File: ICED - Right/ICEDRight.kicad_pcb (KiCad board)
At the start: 2 copper layers, 175.4 x 145.5 mm, 162 parts, among them P1 FLASH_HDR, P2 USB3_MICRO, P3 CONN_17, P4 USB3_AFEMALE, Q1 TC1264, U1 MK20DX256VLH7, U2 IS31FL3731C, X1 CRYSTAL

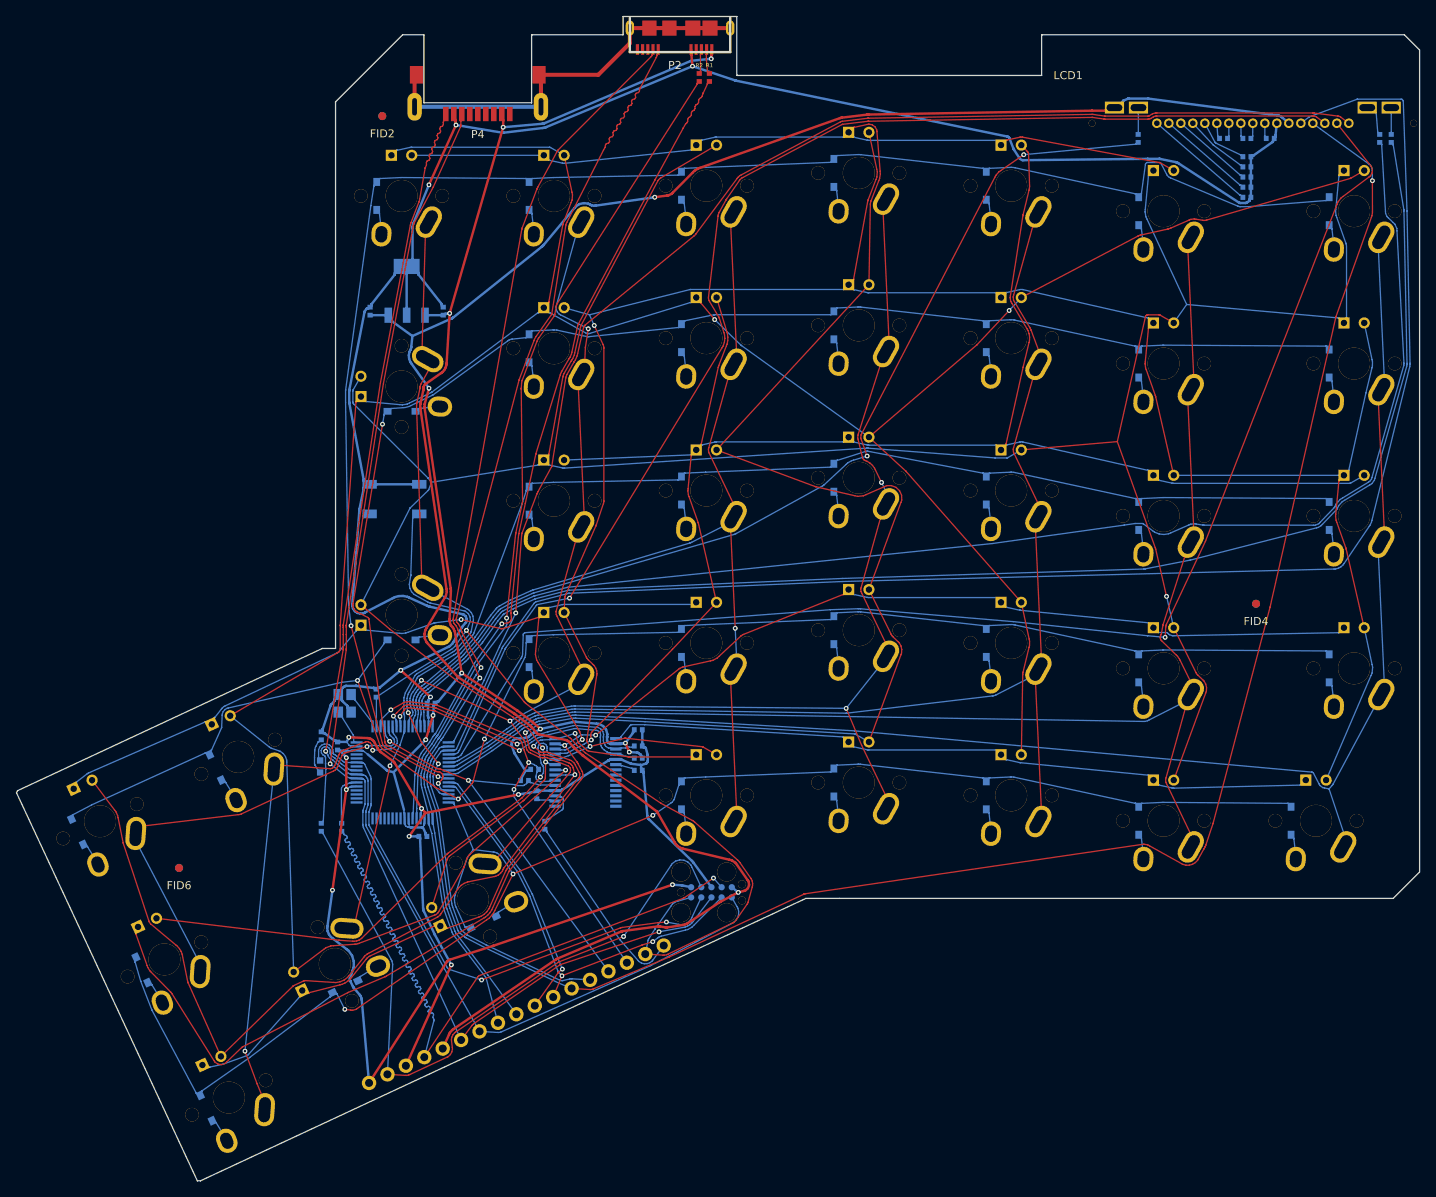
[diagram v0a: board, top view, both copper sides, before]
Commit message: ICED 1.2b, now with 100% more Type C
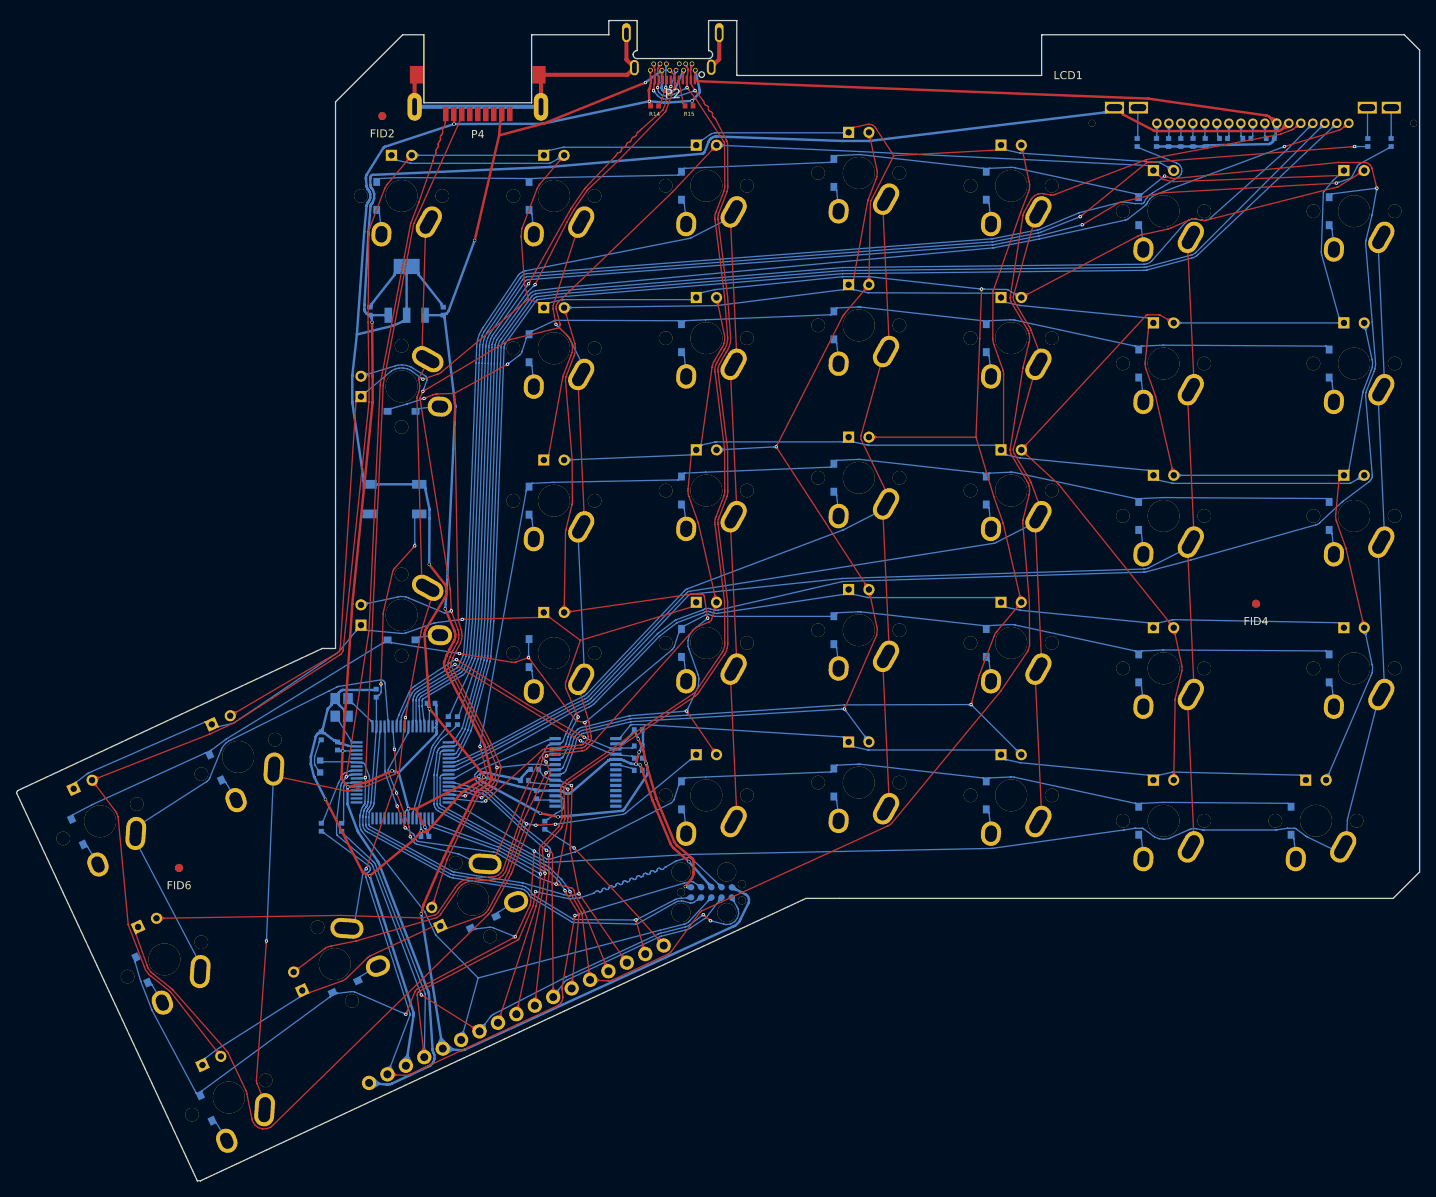
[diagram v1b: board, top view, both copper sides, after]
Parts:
- added R14: 5.1k, prettylib:SMD-1005, F.Cu at (104.0, 53.8)
- added R15: 5.1k, prettylib:SMD-1005, F.Cu at (108.3, 53.8)
- P2: value USB3_MICRO -> USBC; footprint prettylib:USB3_MICROB_STAKES -> prettylib:USB_C_MIDMOUNT_TH_IMPCUT
- R1, R2: moved to B.Cu
- moved R1 86.3 mm to (79.4, 130.7), turned to 180 degrees
- moved R2 86.3 mm to (78.2, 130.7), turned to 180 degrees
- moved C17 13.2 mm to (166.8, 58.4), turned to 0 degrees
- moved C16 11.3 mm to (168.3, 58.4), turned to 0 degrees
- moved C15 9.32 mm to (169.8, 58.4), turned to 0 degrees
- moved C14 7.39 mm to (171.3, 58.4), turned to 0 degrees
- moved P2 7.27 mm to (106.3, 49.9)
- moved C13 5.50 mm to (172.8, 58.4), turned to 0 degrees
- moved R10 1.57 mm to (193.2, 58.4)
- moved X1 0.64 mm to (64.9, 129.0)
- moved R13 0.52 mm to (164.3, 58.4)
- moved R9 0.51 mm to (196.1, 58.4)
- moved C4 0.25 mm to (75.3, 145.2)
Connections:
- net /mcu/PTB18 renamed /Col3
- net /mcu/PTB19 renamed /Col4
- net /mcu/PTB2 renamed /Col1
- net /mcu/PTB3 renamed /Col2
- net /mcu/PTC0 renamed /Col5
- net /mcu/PTC10 renamed /Col7
- net /mcu/PTC11 renamed /Col8
- net /mcu/PTC9 renamed /Col6
- net /mcu/PTD0 renamed /Col9
- net /mcu/PTD1 renamed /Row1
- net /mcu/PTD4 renamed /Row2
- net /mcu/PTD5 renamed /Row3
- net /mcu/PTD6 renamed /Row4
- net /mcu/PTD7 renamed /Row5
- P2 pad 1: +5V -> VSS
- P2 pad 10: (no net) -> /mcu/RX1
- P2 pad 11: /mcu/GND -> /mcu/TX1
- P2 pad 2: Net-(P2-Pad2) -> /mcu/TX1
- P2 pad 3: Net-(P2-Pad3) -> /mcu/RX1
- P2 pad 4: (no net) -> +5V
- P2 pad 5: VSS -> Net-(P2-Pad5)
- P2 pad 6: /mcu/RX1 -> /mcu/USB_DP
- P2 pad 7: /mcu/TX1 -> /mcu/USB_DM
- P2 pad 8: (no net) -> Net-(P2-Pad8)
- P2 pad 9: (no net) -> +5V
- P4 pad 10: /mcu/GND -> /GND
- P4 pad 2: (no net) -> Net-(P4-Pad2)
- P4 pad 3: (no net) -> Net-(P4-Pad3)
- P4 pad 7: (no net) -> Net-(P4-Pad7)
- P4 pad 8: (no net) -> Net-(P4-Pad8)
- P4 pad 9: (no net) -> Net-(P4-Pad9)
- R1 pad 1: Net-(P2-Pad2) -> /mcu/USB_DP
- R1 pad 2: /mcu/USB_DM -> Net-(R1-Pad2)
- R2 pad 1: Net-(P2-Pad3) -> /mcu/USB_DM
- R2 pad 2: /mcu/USB_DP -> Net-(R2-Pad2)
- S39 pad 1: (no net) -> Net-(S39-Pad1)
- U1 pad 10: (no net) -> /mcu/ADC0_DM0
- U1 pad 11: (no net) -> /mcu/ADC1_DP0
- U1 pad 12: (no net) -> /mcu/ADC1_DM0
- U1 pad 13: (no net) -> Net-(U1-Pad13)
- U1 pad 14: (no net) -> Net-(U1-Pad14)
- U1 pad 15: (no net) -> Net-(U1-Pad15)
- U1 pad 16: (no net) -> Net-(U1-Pad16)
- U1 pad 17: (no net) -> Net-(U1-Pad17)
- U1 pad 18: (no net) -> Net-(U1-Pad18)
- U1 pad 19: (no net) -> Net-(U1-Pad19)
- U1 pad 20: (no net) -> Net-(U1-Pad20)
- U1 pad 26: (no net) -> /mcu/PTA4
- U1 pad 28: (no net) -> /mcu/PTA12
- U1 pad 29: (no net) -> /mcu/PTA13
- U1 pad 5: /mcu/USB_DP -> Net-(R1-Pad2)
- U1 pad 6: /mcu/USB_DM -> Net-(R2-Pad2)
- U1 pad 9: (no net) -> /mcu/ADC0_DP0
- U2 pad 10: (no net) -> /mcu/CB4
- U2 pad 11: (no net) -> /mcu/CB5
- U2 pad 12: (no net) -> /mcu/CB6
- U2 pad 13: (no net) -> /mcu/CB7
- U2 pad 14: (no net) -> /mcu/CB8
- U2 pad 15: (no net) -> /mcu/CB9
- U2 pad 7: (no net) -> /mcu/CB1
- U2 pad 8: (no net) -> /mcu/CB2
- U2 pad 9: (no net) -> /mcu/CB3
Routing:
- net /Row1: track 207.7 -> 302.4 mm
- net /ledmatrix/CA2: track 366.3 -> 421.7 mm, vias 3 -> 4
- net /mcu/GND: track 51.4 -> 0.00 mm
- net /GND: track 0.00 -> 45.5 mm
- net /ledmatrix/CA4: track 274.3 -> 311.9 mm
- net /Col5: track 129.5 -> 166.8 mm, vias 1 -> 0
- net VSS: track 367.1 -> 403.3 mm, vias 10 -> 13
- net /mcu/TX1: track 132.9 -> 165.5 mm, vias 1 -> 3
- net /ledmatrix/CA3: track 351.3 -> 383.6 mm
- net /mcu/RX1: track 133.1 -> 164.9 mm, vias 1 -> 3
- net /mcu/MOSI: track 238.3 -> 209.6 mm, vias 0 -> 1
- net /mcu/LCD_KR: track 127.3 -> 152.9 mm, vias 2 -> 0
- net /ledmatrix/CA1: track 361.3 -> 386.3 mm
- net /mcu/MCU_RESET: track 113.7 -> 96.1 mm, vias 1 -> 3
- net /mcu/SDA0: track 54.0 -> 71.0 mm, vias 2 -> 4
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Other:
- board size 175.4 x 145.5 mm -> 175.4 x 145 mm
- net class 4mil added: clearance 0.1016, trace_width 0.1016, via_dia 0.4064, via_drill 0.2032
- net class Default: clearance 0.1524 -> 0.1016; via_dia 0.6096 -> 0.4064; via_drill 0.3048 -> 0.2032
- net class GND: clearance 0.1524 -> 0.1016
- net class Power: clearance 0.1524 -> 0.1016
- rule pad_to_mask_clearance: 0.0762 -> 0.0508
- rule trace_clearance: 0.1524 -> 0.1016
- rule via_min_drill: 0.3048 -> 0.2032
- rule via_min_size: 0.508 -> 0.4064
- board text added: "ICED-R Rev 1.2b Batch __"
- board text removed: "ICED-R Rev 1.1d Batch __"
